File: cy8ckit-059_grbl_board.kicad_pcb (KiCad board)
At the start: 2 copper layers, 78.7 x 64.1 mm, 24 parts, among them IC1 CY8CKIT-059, J1 Connector:Conn_01x04_Male, J10 Conn_02x01, J11 Conn_02x01, J12 Conn_02x04_Odd_Even, J13 Conn_02x03_Odd_Even, J2 Connector:Conn_01x04_Male, J3 Connector:Conn_01x04_Male, J4 Conn_02x03_Odd_Even, J5 Conn_02x03_Odd_Even, J6 Conn_02x03_Odd_Even, J7 Conn_02x02_Odd_Even, J8 Conn_02x05_Odd_Even, J9 Screw_Terminal_01x02

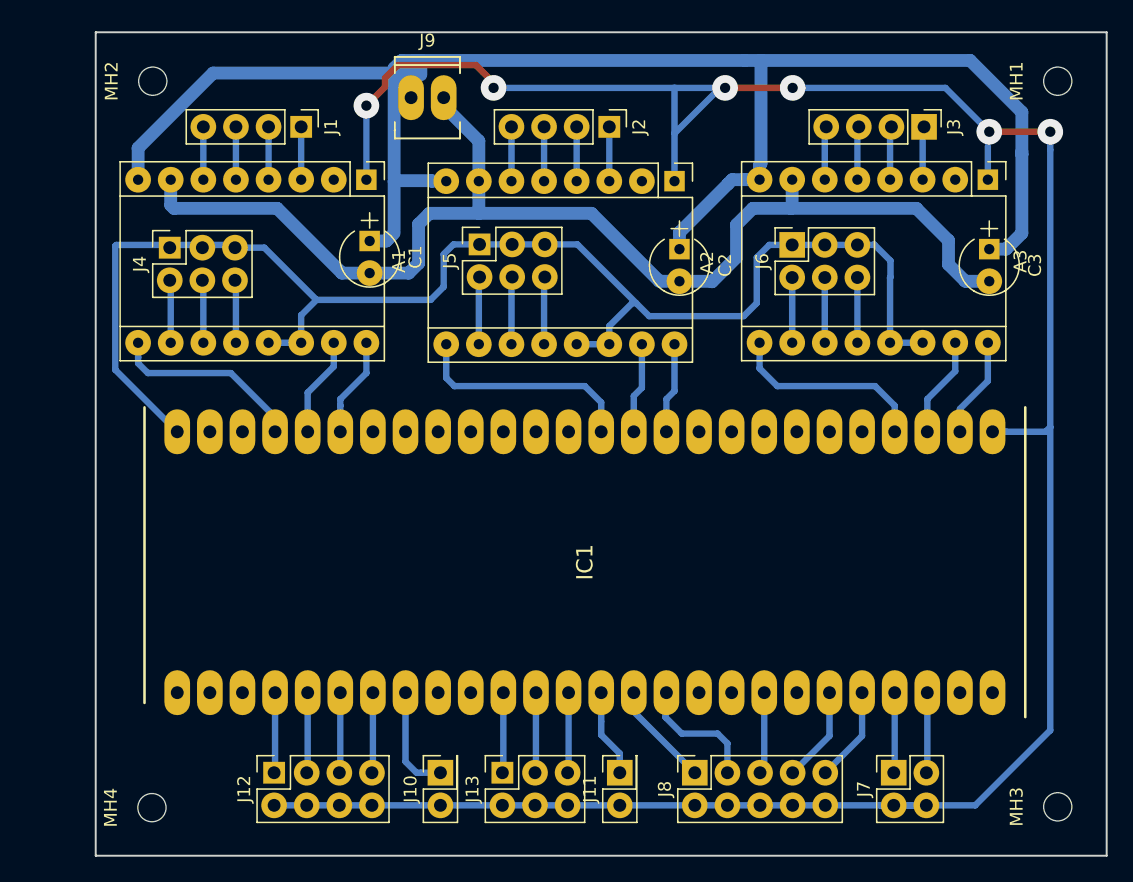
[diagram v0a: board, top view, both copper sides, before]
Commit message: V2.0
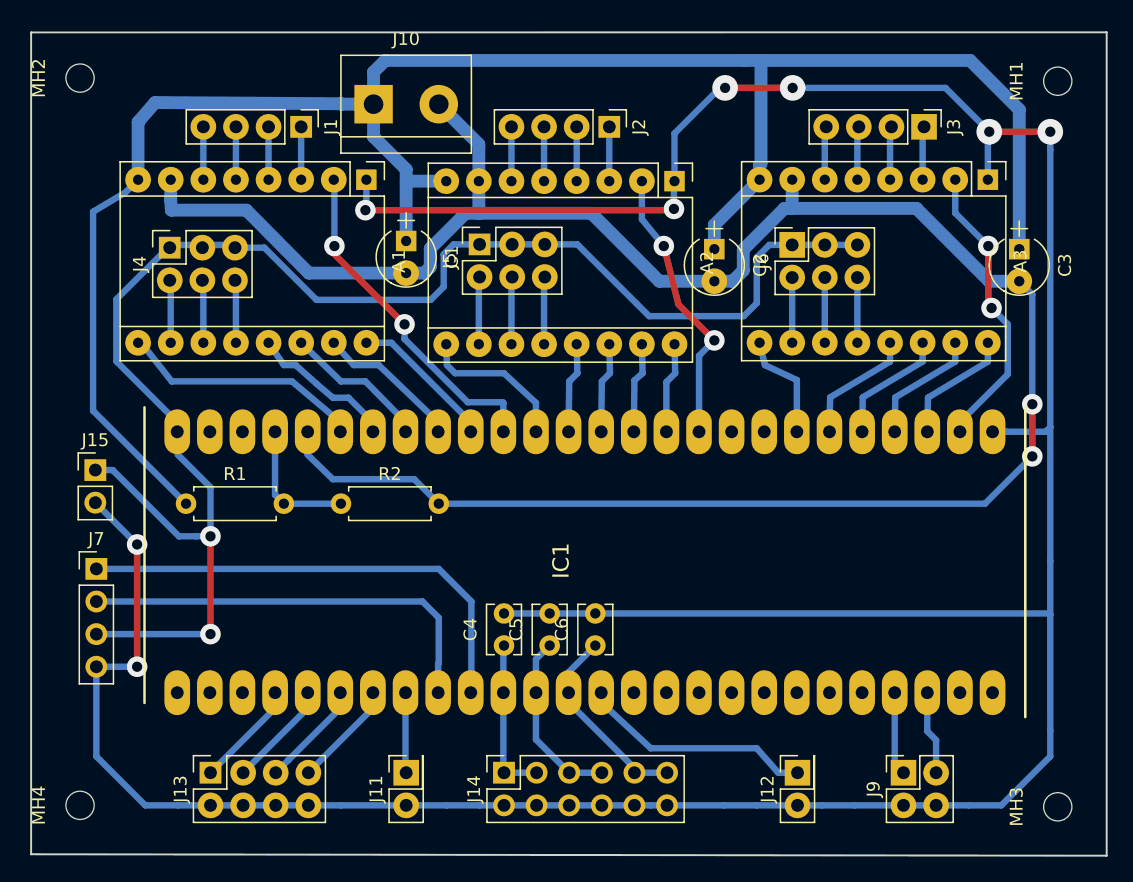
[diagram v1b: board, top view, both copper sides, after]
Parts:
- removed the J13 at (106.7, 110.5)
- removed J8: Conn_02x05_Odd_Even, Socket_Strips:Socket_Strip_Straight_2x05_Pitch2.54mm
- removed the J9 at (100.8, 57.9)
- added C4: 100nF, Capacitors_THT:C_Disc_D3.8mm_W2.6mm_P2.50mm, F.Cu at (106.8, 100.6)
- added C5: 100nF, Capacitors_THT:C_Disc_D3.8mm_W2.6mm_P2.50mm, F.Cu at (110.4, 100.6)
- added C6: 100nF, Capacitors_THT:C_Disc_D3.8mm_W2.6mm_P2.50mm, F.Cu at (113.9, 100.6)
- added J10: Screw_Terminal_01x02, Connectors_Terminal_Blocks:TerminalBlock_bornier-2_P5.08mm, F.Cu at (96.6, 58.4)
- added J14: Conn_02x06_Odd_Even, Socket_Strips:Socket_Strip_Straight_2x06_Pitch2.54mm, F.Cu at (106.8, 110.5)
- added J15: Conn_01x02_Male, Socket_Strips:Socket_Strip_Straight_1x02_Pitch2.54mm, F.Cu at (75.0, 86.9)
- added J7: Conn_01x04_Male, Socket_Strips:Socket_Strip_Straight_1x04_Pitch2.54mm, F.Cu at (75.1, 94.6)
- added R1: R, Resistors_THT:R_Axial_DIN0207_L6.3mm_D2.5mm_P7.62mm_Horizontal, F.Cu at (82.0, 89.5)
- added R2: R, Resistors_THT:R_Axial_DIN0207_L6.3mm_D2.5mm_P7.62mm_Horizontal, F.Cu at (94.1, 89.5)
- moved J12 13.8 mm to (129.7, 110.5)
- moved MH2 5.67 mm to (73.8, 56.4)
- moved MH4 5.60 mm to (73.8, 113.0)
- moved J13 4.96 mm to (83.9, 110.5)
- moved C1 2.84 mm to (99.2, 69.1)
- moved C2 2.72 mm to (123.2, 69.7)
- moved J11 2.67 mm to (99.2, 110.5)
- moved C3 2.34 mm to (146.9, 69.7)
- moved J9 0.76 mm to (137.9, 110.5)
- renumbered J10 to J11, J11 to J12, J12 to J13, J7 to J9
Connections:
- A1 pad 13: +5V -> /reset_x
- A1 pad 14: +5V -> /sleep_x
- A1 pad 2: (no net) -> /fault_x
- A1 pad 9: /step_enable_x -> /enable_x
- A2 pad 13: +5V -> /reset_y
- A2 pad 14: +5V -> /sleep_y
- A2 pad 2: (no net) -> /fault_y
- A2 pad 9: /step_enable_y -> /enable_y
- A3 pad 13: +5V -> /reset_z
- A3 pad 14: +5V -> /sleep_z
- A3 pad 2: (no net) -> /fault_z
- A3 pad 9: /step_enable_z -> /enable_z
- IC1 pad 10: (no net) -> /uart_rx
- IC1 pad 15: /lcd_i2c_sda -> (no net)
- IC1 pad 16: /lcd_i2c_scl -> (no net)
- IC1 pad 19: /encoder_A -> (no net)
- IC1 pad 21: /encoder_B -> (no net)
- IC1 pad 22: /encoder_switch -> (no net)
- IC1 pad 28: /dir_z -> /fault_z
- IC1 pad 29: /step_z -> /dir_z
- IC1 pad 30: /step_enable_z -> /step_z
- IC1 pad 31: (no net) -> /sleep_z
- IC1 pad 32: (no net) -> /reset_z
- IC1 pad 33: (no net) -> /enable_z
- IC1 pad 36: (no net) -> /fault_y
- IC1 pad 39: /step_enable_y -> /sleep_y
- IC1 pad 40: (no net) -> /reset_y
- IC1 pad 41: (no net) -> /enable_y
- IC1 pad 42: (no net) -> /fault_x
- IC1 pad 43: (no net) -> /dir_x
- IC1 pad 44: (no net) -> /step_x
- IC1 pad 45: (no net) -> /sleep_x
- IC1 pad 46: (no net) -> /reset_x
- IC1 pad 47: /dir_x -> /enable_x
- IC1 pad 48: /step_x -> GND
- IC1 pad 49: /step_enable_x -> /motor_voltage
- IC1 pad 9: (no net) -> /uart_tx
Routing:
- net GND: track 93.5 -> 169.3 mm, vias 0 -> 2
- net GNDD: track 196.4 -> 266.9 mm, vias 6 -> 8
- net /uart_rx: track 0.00 -> 37.4 mm
- net /uart_tx: track 0.00 -> 33.0 mm
- net /fault_x: track 0.00 -> 26.7 mm, vias 0 -> 2
- net /fault_z: track 0.00 -> 23.2 mm, vias 0 -> 2
- net /fault_y: track 0.00 -> 22.0 mm, vias 0 -> 2
- net +36V: track 130.7 -> 150.3 mm
- net /enable_x: track 0.00 -> 19.1 mm
- net /step_enable_y: track 17.8 -> 0.00 mm
- net /step_enable_z: track 15.8 -> 0.00 mm
- net /step_enable_x: track 15.1 -> 0.00 mm
- net /enable_y: track 0.00 -> 12.0 mm
- net /reset_x: track 0.00 -> 11.5 mm
- net /spindle_pwm: track 6.84 -> 18.3 mm
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- removed copper zone on B.Cu, net +36V
- removed copper zone on B.Cu, net GNDD
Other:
- board size 78.7 x 64.1 mm -> 83.8 x 64.1 mm
- net class Power added: clearance 0.3, trace_width 1, via_dia 1.6, via_drill 0.8
